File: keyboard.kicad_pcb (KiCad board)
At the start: 2 copper layers, 108.2 x 96.2 mm, 117 parts, among them J2 TYPE-C-31-M-12, U1 ATmega32U4-A, Y1 Crystal_GND24_Small

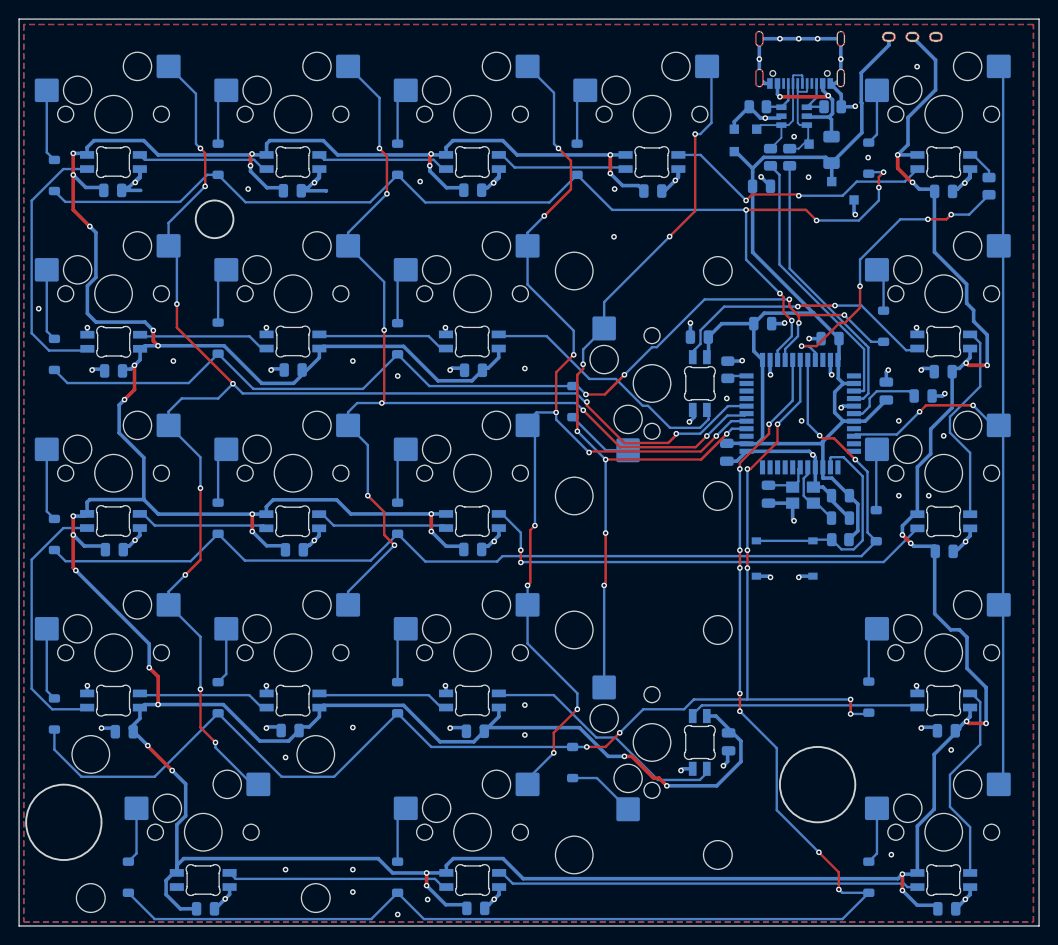
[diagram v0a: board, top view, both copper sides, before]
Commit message: update
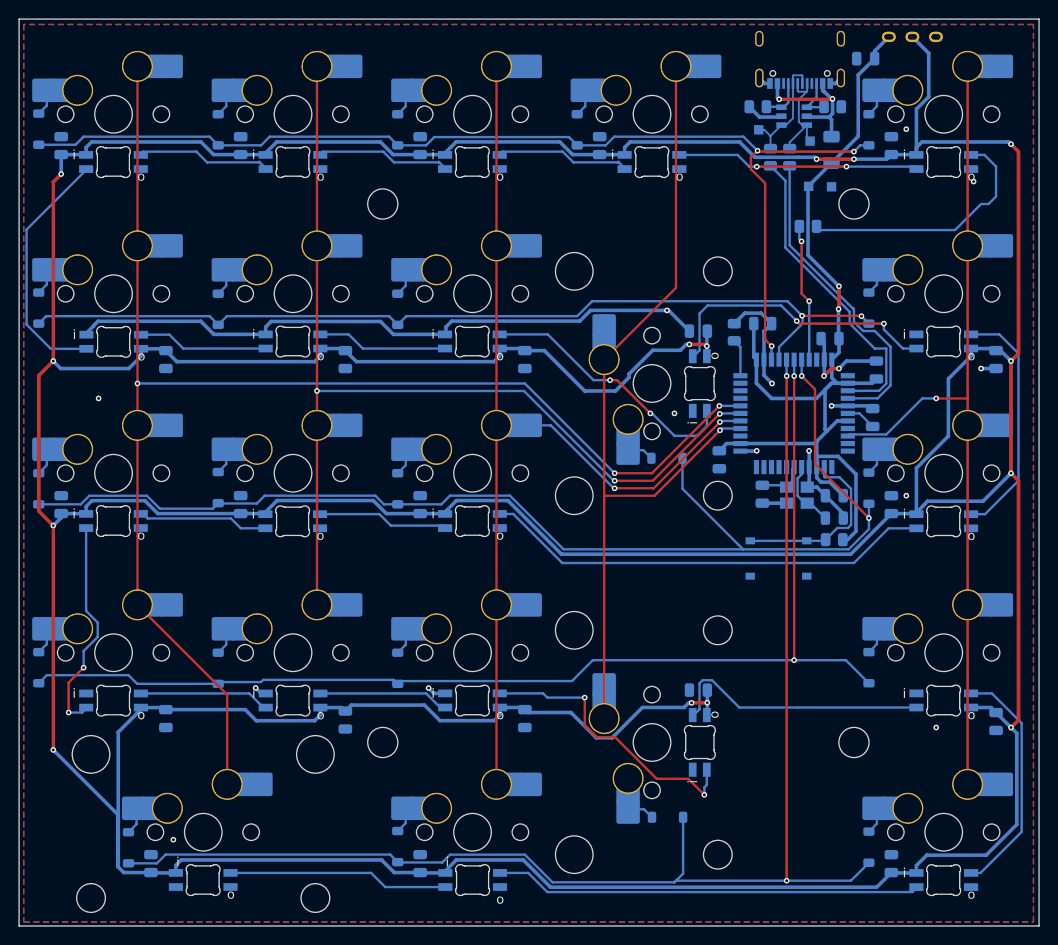
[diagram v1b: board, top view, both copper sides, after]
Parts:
- removed 5V+ (x2), GND (x2): Power, TestPoint:TestPoint_Pad_1.0x1.0mm
- removed D+: D+, TestPoint:TestPoint_Pad_1.0x1.0mm
- removed D-: D-, TestPoint:TestPoint_Pad_1.0x1.0mm
- added 5V+2: Power, TestPoint:TestPoint_Pad_1.0x1.0mm, B.Cu at (242.1, 77.5)
- added D+1: D+, TestPoint:TestPoint_Pad_1.0x1.0mm, B.Cu at (242.2, 72.7)
- added D-1: D-, TestPoint:TestPoint_Pad_1.0x1.0mm, B.Cu at (236.8, 71.5)
- added GND1: Power, TestPoint:TestPoint_Pad_1.0x1.0mm, B.Cu at (244.5, 77.5)
- added H1: MountingHole, MountingHole:MountingHole_3.2mm_M3, F.Cu at (196.8, 79.4)
- added H2: MountingHole, MountingHole:MountingHole_3.2mm_M3, F.Cu at (196.8, 136.5)
- added H3: MountingHole, MountingHole:MountingHole_3.2mm_M3, F.Cu at (246.9, 136.5)
- added H4: MountingHole, MountingHole:MountingHole_3.2mm_M3, F.Cu at (246.9, 79.4)
- added H5: MountingHole, marbastlib-mx:STAB_MX_2u, F.Cu at (225.4, 98.4)
- added H6: MountingHole, marbastlib-mx:STAB_MX_2u, F.Cu at (225.4, 136.5)
- added H7: MountingHole, marbastlib-mx:STAB_MX_2u, F.Cu at (177.8, 146.0)
- Custom-1, Custom-2, Custom-3, Custom-4, Custom-5, Key_*1, Key_-1, Key_/1, Key_1, Key_2, Key_3, Key_4, Key_5, Key_6, Key_7, Key_8, Key_9, Key_del1, NumLock1: footprint MX_keys:MX-Hotswap-1U -> marbastlib-mx:SW_MX_HS_S_CPG151101S11_1u
- Key_+1, Key_0, Key_enter1: footprint Button_Switch_Keyboard:MX-Hotswap-2U-ReversedStabilizers -> marbastlib-mx:SW_MX_HS_S_CPG151101S11_1u
- U10, U11, U12, U13, U14, U15, U16, U17, U18, U2, U20, U21, U22, U23, U24, U3, U4, U5, U6, U7, U8, U9: moved to B.Cu
- moved C31 124.1 mm to (162.7, 73.2), turned to -90 degrees
- moved C13 109.4 mm to (261.9, 134.3), turned to 90 degrees
- moved C30 84.7 mm to (181.8, 73.2), turned to -90 degrees
- moved C29 84.1 mm to (200.8, 73.2), turned to -90 degrees
- moved C17 80.7 mm to (172.2, 149.4), turned to -90 degrees
- moved C28 80.1 mm to (219.9, 73.2), turned to -90 degrees
- moved C12 76.8 mm to (261.9, 95.9), turned to 90 degrees
- moved C18 76.2 mm to (200.8, 149.4), turned to -90 degrees
- moved C20 71.6 mm to (250.8, 149.4), turned to -90 degrees
- moved C9 71.4 mm to (211.9, 134.0), turned to 90 degrees
- moved C10 64.9 mm to (192.9, 134.1), turned to 90 degrees
- moved C11 64.8 mm to (173.8, 134.0), turned to 90 degrees
- moved C19 63.8 mm to (230.3, 131.0), turned to 0 degrees
- moved C27 61.7 mm to (250.8, 73.2), turned to -90 degrees
- moved C22 49.9 mm to (230.3, 92.9)
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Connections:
- C10 pad 2: +5V -> LEDP
- C11 pad 2: +5V -> LEDP
- C12 pad 2: +5V -> LEDP
- C13 pad 2: +5V -> LEDP
- C14 pad 2: +5V -> LEDP
- C15 pad 2: +5V -> LEDP
- C16 pad 2: +5V -> LEDP
- C17 pad 2: +5V -> LEDP
- C18 pad 2: +5V -> LEDP
- C19 pad 2: +5V -> LEDP
- C20 pad 2: +5V -> LEDP
- C21 pad 2: +5V -> LEDP
- C22 pad 2: +5V -> LEDP
- C23 pad 2: +5V -> LEDP
- C24 pad 2: +5V -> LEDP
- C25 pad 2: +5V -> LEDP
- C27 pad 2: +5V -> LEDP
- C28 pad 2: +5V -> LEDP
- C29 pad 2: +5V -> LEDP
- C30 pad 2: +5V -> LEDP
- C31 pad 2: +5V -> LEDP
- C9 pad 2: +5V -> LEDP
- D12 pad 1: X1 -> X2
- D16 pad 1: X3 -> X4
- SW1 pad 2: +5V -> LEDP
- U10 pad 1: +5V -> LEDP
- U11 pad 1: +5V -> LEDP
- U12 pad 1: +5V -> LEDP
- U13 pad 1: +5V -> LEDP
- U14 pad 1: +5V -> LEDP
- U15 pad 1: +5V -> LEDP
- U16 pad 1: +5V -> LEDP
- U17 pad 1: +5V -> LEDP
- U18 pad 1: +5V -> LEDP
- U2 pad 1: +5V -> LEDP
- U20 pad 1: +5V -> LEDP
- U21 pad 1: +5V -> LEDP
- U22 pad 1: +5V -> LEDP
- U23 pad 1: +5V -> LEDP
- U24 pad 1: +5V -> LEDP
- U3 pad 1: +5V -> LEDP
- U4 pad 1: +5V -> LEDP
- U5 pad 1: +5V -> LEDP
- U6 pad 1: +5V -> LEDP
- U7 pad 1: +5V -> LEDP
- U8 pad 1: +5V -> LEDP
- U9 pad 1: +5V -> LEDP
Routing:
- net LEDP: track 0.00 -> 688.6 mm, vias 0 -> 14
- net +5V: track 707.6 -> 104.1 mm, vias 38 -> 2
- net GND: track 147.8 -> 121.9 mm, vias 83 -> 17
- net LED_DATA_IN: track 3.70 -> 27.1 mm
- net X3: track 141.9 -> 123.1 mm, vias 8 -> 2
- net Net-(U1-PF0): track 32.1 -> 14.7 mm, vias 4 -> 2
- net X2: track 116.4 -> 128.5 mm
- net Y2: track 114.1 -> 104.3 mm, vias 10 -> 2
- net X1: track 106.6 -> 97.3 mm, vias 5 -> 2
- net X0: track 120.3 -> 115.0 mm, vias 6 -> 3
- net X4: track 149.4 -> 144.3 mm, vias 8 -> 2
- net Net-(D1-A): track 7.73 -> 2.83 mm
- net Net-(D6-A): track 7.73 -> 2.83 mm
- net Net-(D3-A): track 7.66 -> 2.77 mm
- net Net-(U1-UCAP): track 8.09 -> 3.21 mm
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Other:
- outline, holes or cut-outs redrawn
- rule pad_to_mask_clearance: 0.038 -> 0
